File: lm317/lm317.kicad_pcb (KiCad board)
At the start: 2 copper layers, 49.5 x 20.5 mm, 11 parts, among them J1 INPUT, J2 OUTPUT, U1 LM317L_TO92

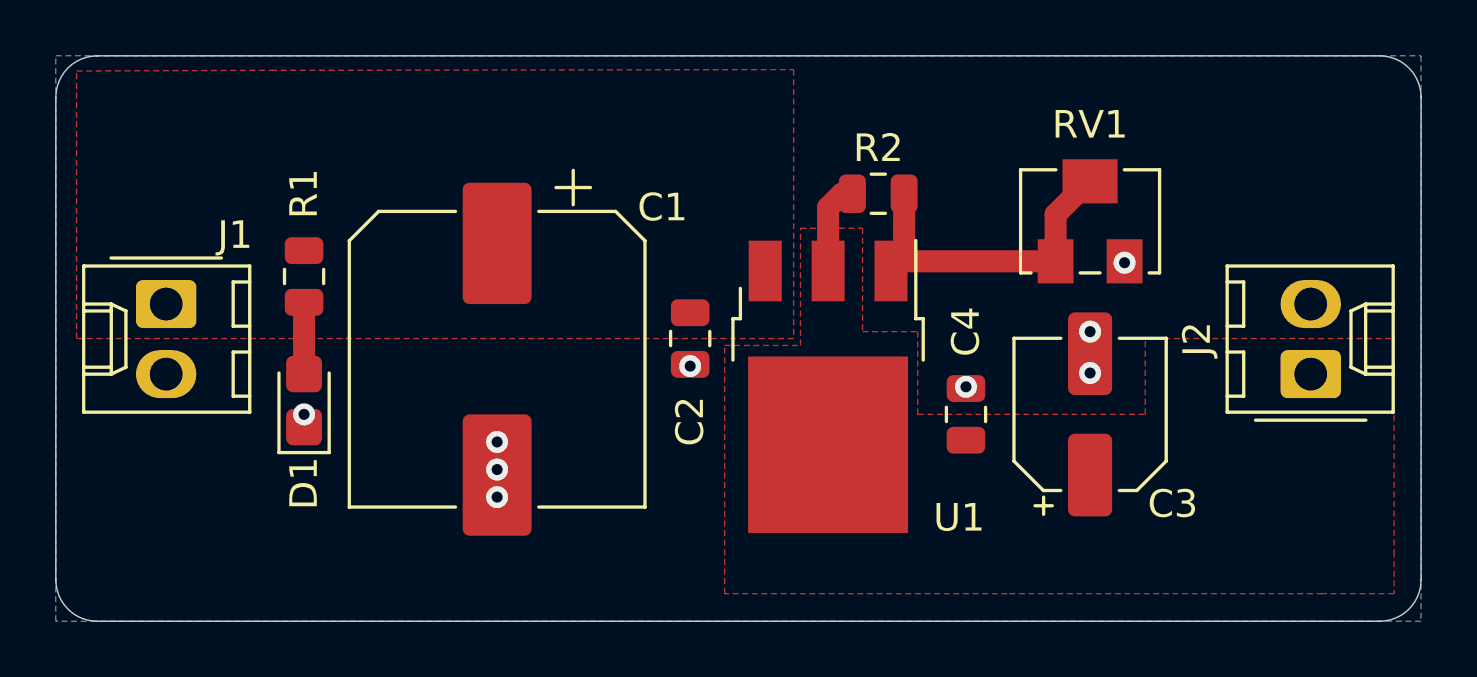
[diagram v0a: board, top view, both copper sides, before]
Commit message: update files
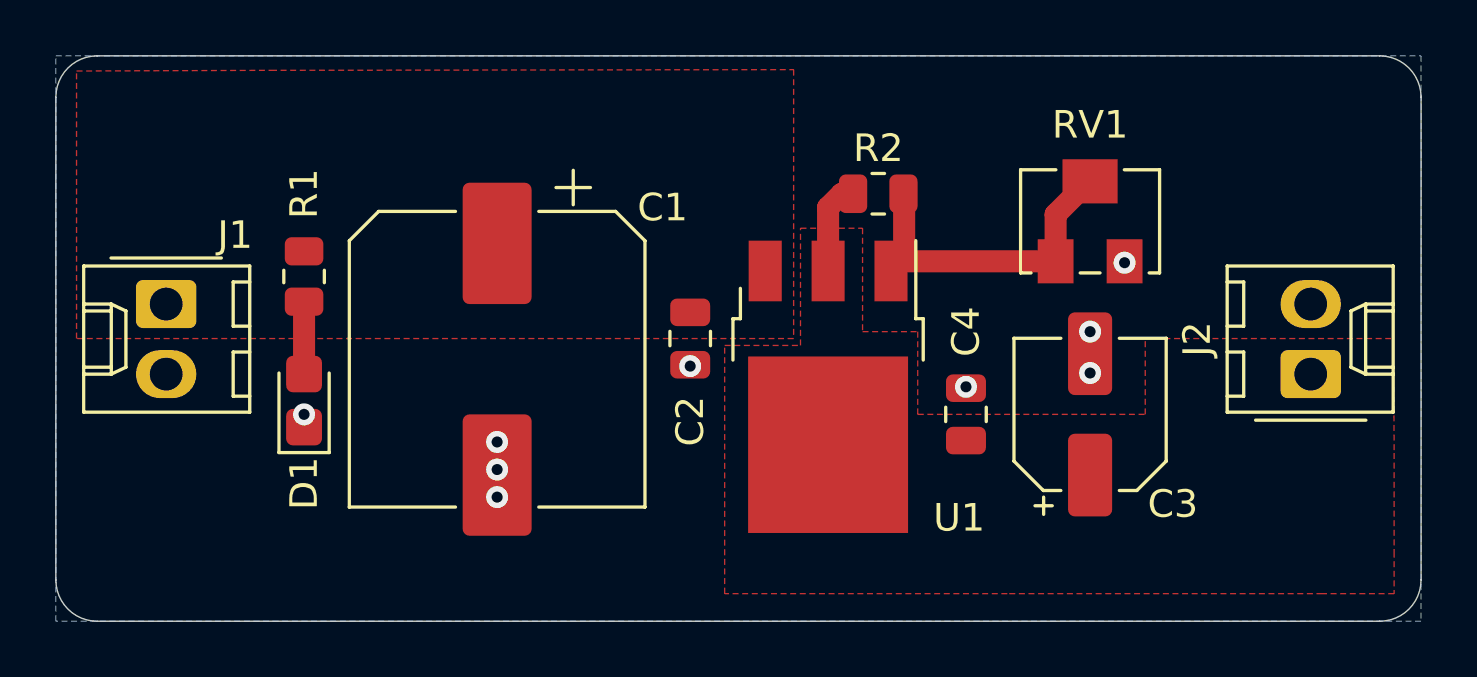
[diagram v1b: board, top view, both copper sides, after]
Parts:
- C3: value 100uF/25V -> 0.1uF/50V
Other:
- net class Default removed
